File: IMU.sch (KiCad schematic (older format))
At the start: 23 parts, among them U3 ICM-20948, U4 MPU-9250, U5 LSM6DS3, U7 LP5907MFX-1.8, U8 LP5907MFX-3.3

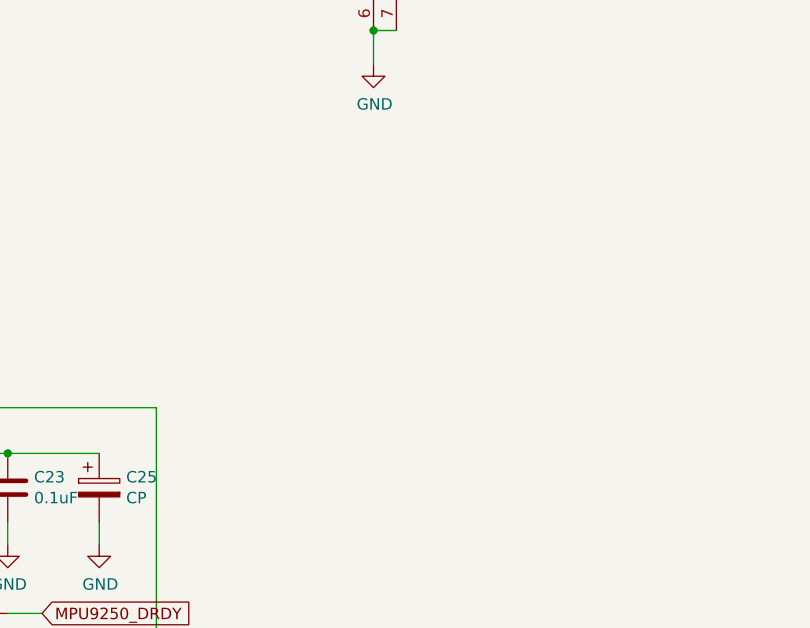
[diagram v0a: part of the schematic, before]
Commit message: finish board
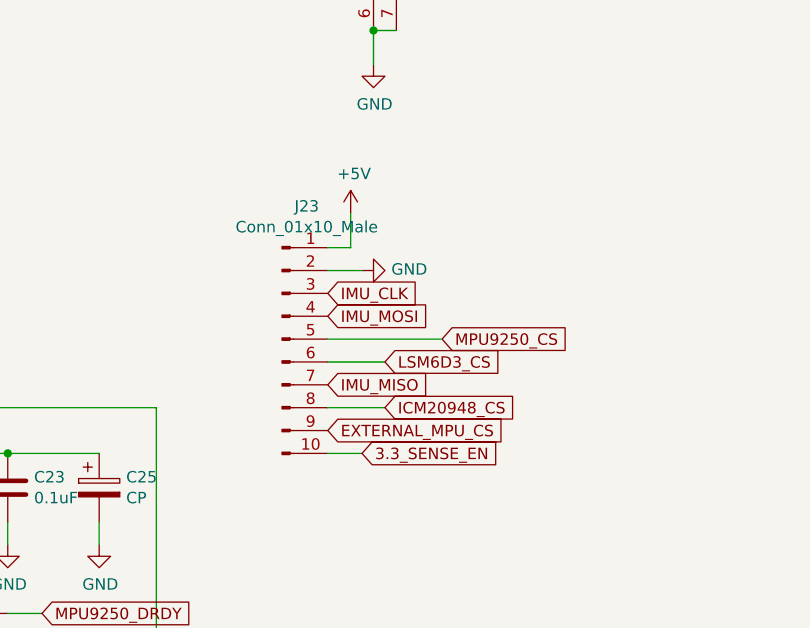
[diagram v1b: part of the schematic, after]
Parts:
- added J23: Conn_01x10_Male, Connector_PinHeader_2.54mm:PinHeader_1x10_P2.54mm_Vertical, symbol Connector:Conn_01x10_Male
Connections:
- net +5V: now also J23.1 (Pin_1)
- net 3.3_SENSE_EN: now also J23.10 (Pin_10)
- net GND: now also J23.2 (Pin_2)
- net ICM20948_CS: now also J23.8 (Pin_8)
- net IMU_CLK: now also J23.3 (Pin_3)
- net IMU_MISO: now also J23.7 (Pin_7)
- net IMU_MOSI: now also J23.4 (Pin_4)
- net LSM6D3_CS: now also J23.6 (Pin_6)
- net MPU9250_CS: now also J23.5 (Pin_5)
- new net EXTERNAL_MPU_CS: J23.9 (Pin_9)
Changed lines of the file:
@@
 Wire Wire Line
 	1900 5550 2400 5550
+$Comp
+L power:+5V #PWR?
+U 1 1 5F649538
+P 5450 3350
+AR Path="/5F3218EE/5F649538" Ref="#PWR?"  Part="1"
+AR Path="/5F649538" Ref="#PWR?"  Part="1"
+AR Path="/5F584BC5/5F649538" Ref="#PWR0188"  Part="1"
+AR Path="/5F5AF088/5F649538" Ref="#PWR?"  Part="1"
+F 0 "#PWR0188" H 5450 3200 50  0001 C CNN
+F 1 "+5V" H 5465 3523 50  0000 C CNN
+F 2 "" H 5450 3350 50  0001 C CNN
+F 3 "" H 5450 3350 50  0001 C CNN
+	1    5450 3350
+	1    0    0    -1
+$EndComp
+Wire Wire Line
+	5350 3500 5450 3500
+Wire Wire Line
+	5450 3500 5450 3350
+$Comp
+L power:GND #PWR0189
+U 1 1 5F65131E
+P 5500 3600
+F 0 "#PWR0189" H 5500 3350 50  0001 C CNN
+F 1 "GND" V 5505 3472 50  0000 R CNN
+F 2 "" H 5500 3600 50  0001 C CNN
+F 3 "" H 5500 3600 50  0001 C CNN
+	1    5500 3600
+	0    -1   -1   0
+$EndComp
+Wire Wire Line
+	5350 3600 5500 3600
+$Comp
+L Connector:Conn_01x10_Male J23
+U 1 1 5F659907
+P 5150 3900
+F 0 "J23" H 5258 4481 50  0000 C CNN
+F 1 "Conn_01x10_Male" H 5258 4390 50  0000 C CNN
+F 2 "Connector_PinHeader_2.54mm:PinHeader_1x10_P2.54mm_Vertical" H 5150 3900 50  0001 C CNN
+F 3 "~" H 5150 3900 50  0001 C CNN
+	1    5150 3900
+	1    0    0    -1
+$EndComp
+Text GLabel 5350 3800 2    50   Input ~ 0
+IMU_MOSI
+Text GLabel 5350 4100 2    50   Input ~ 0
+IMU_MISO
+Text GLabel 5350 3700 2    50   Input ~ 0
+IMU_CLK
+Text GLabel 5350 4300 2    50   Input ~ 0
+EXTERNAL_MPU_CS
+Text GLabel 5600 4200 2    50   Input ~ 0
+ICM20948_CS
+Wire Wire Line
+	5600 4200 5350 4200
+Text GLabel 5600 4000 2    50   Input ~ 0
+LSM6D3_CS
+Wire Wire Line
+	5600 4000 5350 4000
+Text GLabel 5850 3900 2    50   Input ~ 0
+MPU9250_CS
+Wire Wire Line
+	5850 3900 5350 3900
+Text GLabel 5500 4400 2    50   Input ~ 0
+3.3_SENSE_EN
+Wire Wire Line
+	5350 4400 5500 4400
 $EndSCHEMATC
